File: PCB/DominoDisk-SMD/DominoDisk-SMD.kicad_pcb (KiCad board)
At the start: 4 copper layers, 44 x 32.6 mm, 31 parts, among them J1 Daisy port out, J2 ICSP_ISP6, J3 Daisy port in, J4 UART, K1 TF-104 MicroSD card holder, U1 PC817C-S, U2 ATmega328P-AU, U3 TXB0104PWR level shifter, U4 SE5218ALG voltage regulator, Y1 CSTNE16M0V530000R0 Resonator

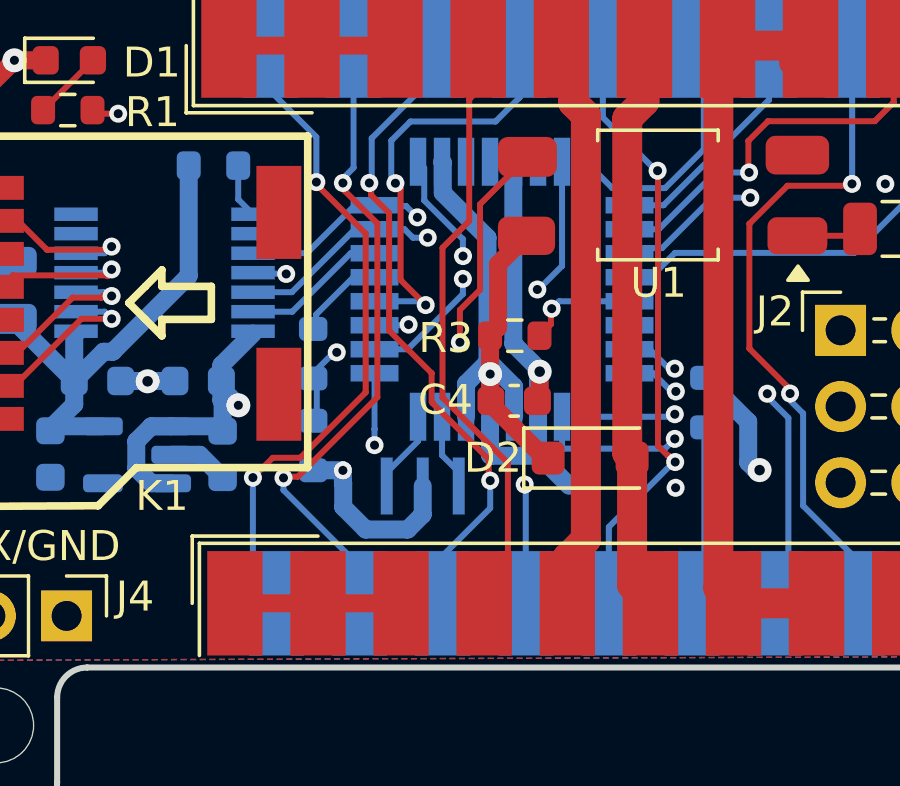
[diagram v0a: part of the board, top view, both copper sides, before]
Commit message: OCD
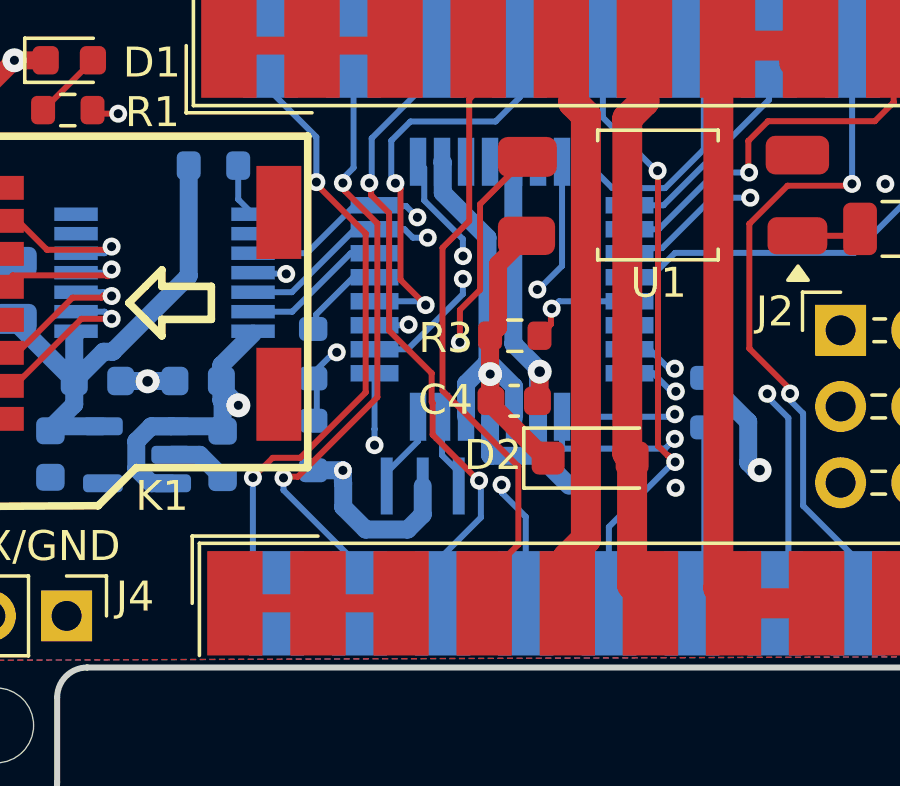
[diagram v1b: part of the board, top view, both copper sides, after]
